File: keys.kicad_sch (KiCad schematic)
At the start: 168 parts, among them SW1 RotaryEncoder_Switch, U11 SLSS49E-3, U12 SLSS49E-3, U13 SLSS49E-3, U14 SLSS49E-3, U15 SLSS49E-3, U16 SLSS49E-3, U17 SLSS49E-3, U18 SLSS49E-3, U19 SLSS49E-3, U2 SLSS49E-3, U20 SLSS49E-3, U21 SLSS49E-3, U22 SLSS49E-3, U23 SLSS49E-3, U24 SLSS49E-3, U25 SLSS49E-3, U26 SLSS49E-3, U27 SLSS49E-3, U28 SLSS49E-3, U29 SLSS49E-3, U30 SLSS49E-3, U31 SLSS49E-3, U32 SLSS49E-3, U33 SLSS49E-3, U34 SLSS49E-3, U35 SLSS49E-3, U36 SLSS49E-3, U37 SLSS49E-3, U38 SLSS49E-3, U39 SLSS49E-3, U4 SLSS49E-3, U40 SLSS49E-3, U41 SLSS49E-3, U42 SLSS49E-3, U43 SLSS49E-3, U44 SLSS49E-3, U45 SLSS49E-3, U46 SLSS49E-3, U47 SLSS49E-3, U48 SLSS49E-3, U49 SLSS49E-3, U50 SLSS49E-3, U51 SLSS49E-3, U52 SLSS49E-3, U53 SLSS49E-3, U54 SLSS49E-3, U55 SLSS49E-3, U56 SLSS49E-3, U57 SLSS49E-3, U58 SLSS49E-3, U59 SLSS49E-3, U60 SLSS49E-3, U61 SLSS49E-3, U62 SLSS49E-3, U63 SLSS49E-3, U64 SLSS49E-3, U65 SLSS49E-3, U66 SLSS49E-3, U67 SLSS49E-3, U68 SLSS49E-3, U69 SLSS49E-3, U70 SLSS49E-3, U71 SLSS49E-3, U72 SLSS49E-3, U73 SLSS49E-3, U74 SLSS49E-3, U75 SLSS49E-3, U76 SLSS49E-3, U77 SLSS49E-3, U78 SLSS49E-3, U79 SLSS49E-3, U80 SLSS49E-3, U81 SLSS49E-3, U82 SLSS49E-3, U83 SLSS49E-3, U84 SLSS49E-3, U85 SLSS49E-3, U86 SLSS49E-3, U87 SLSS49E-3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

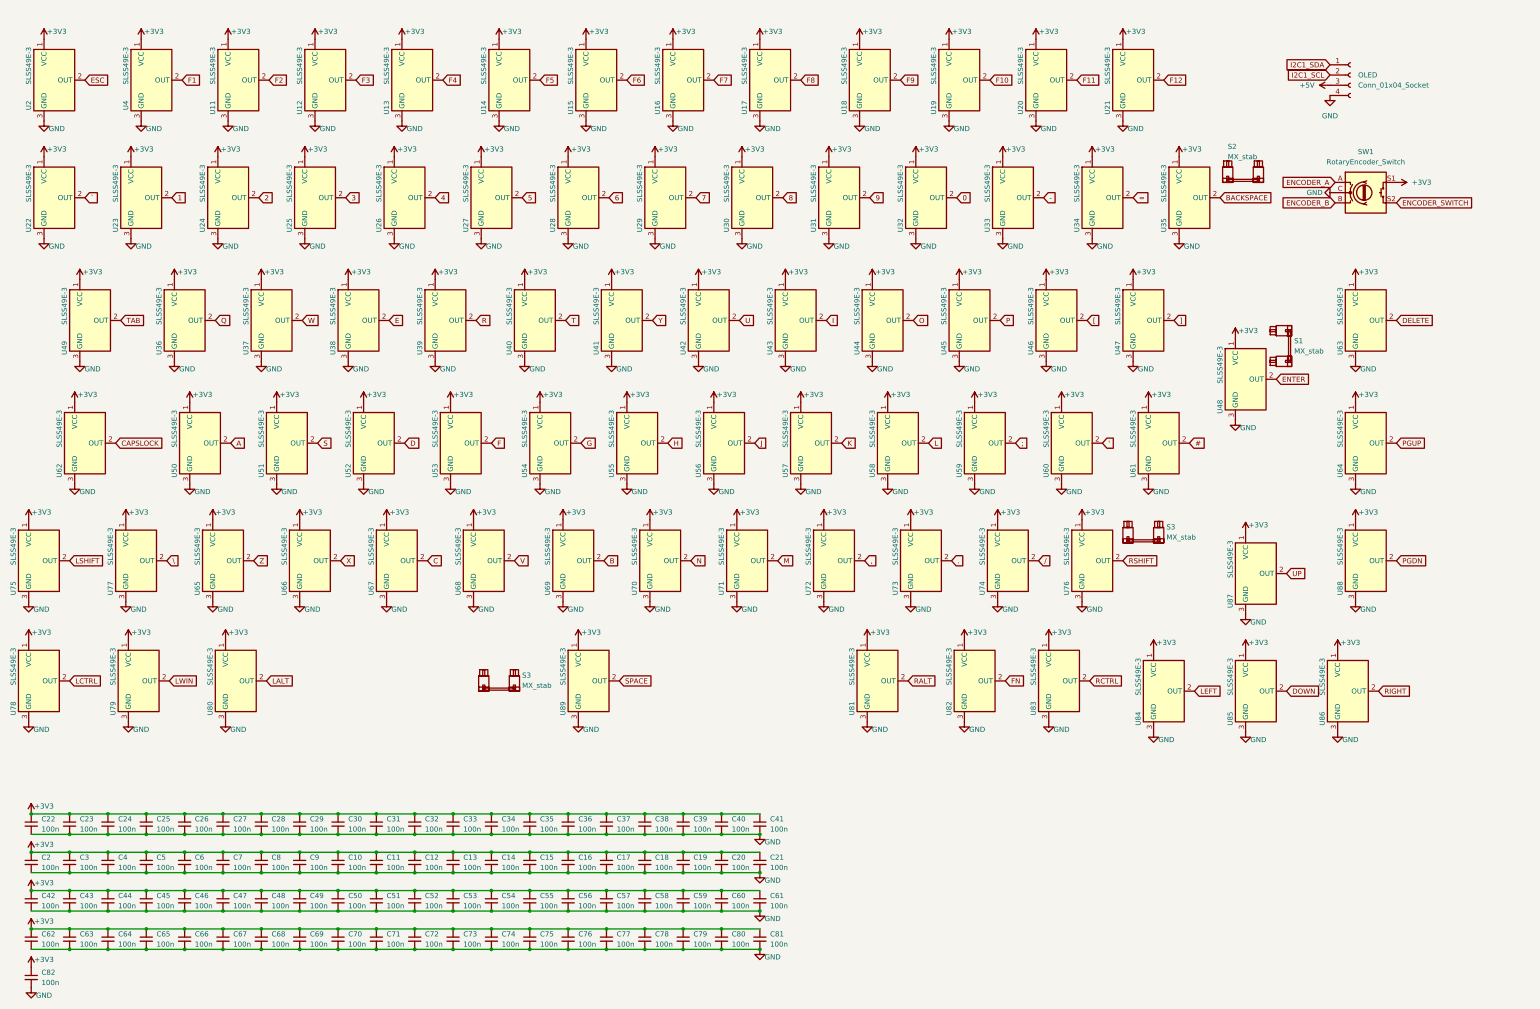
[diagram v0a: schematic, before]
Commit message: bus
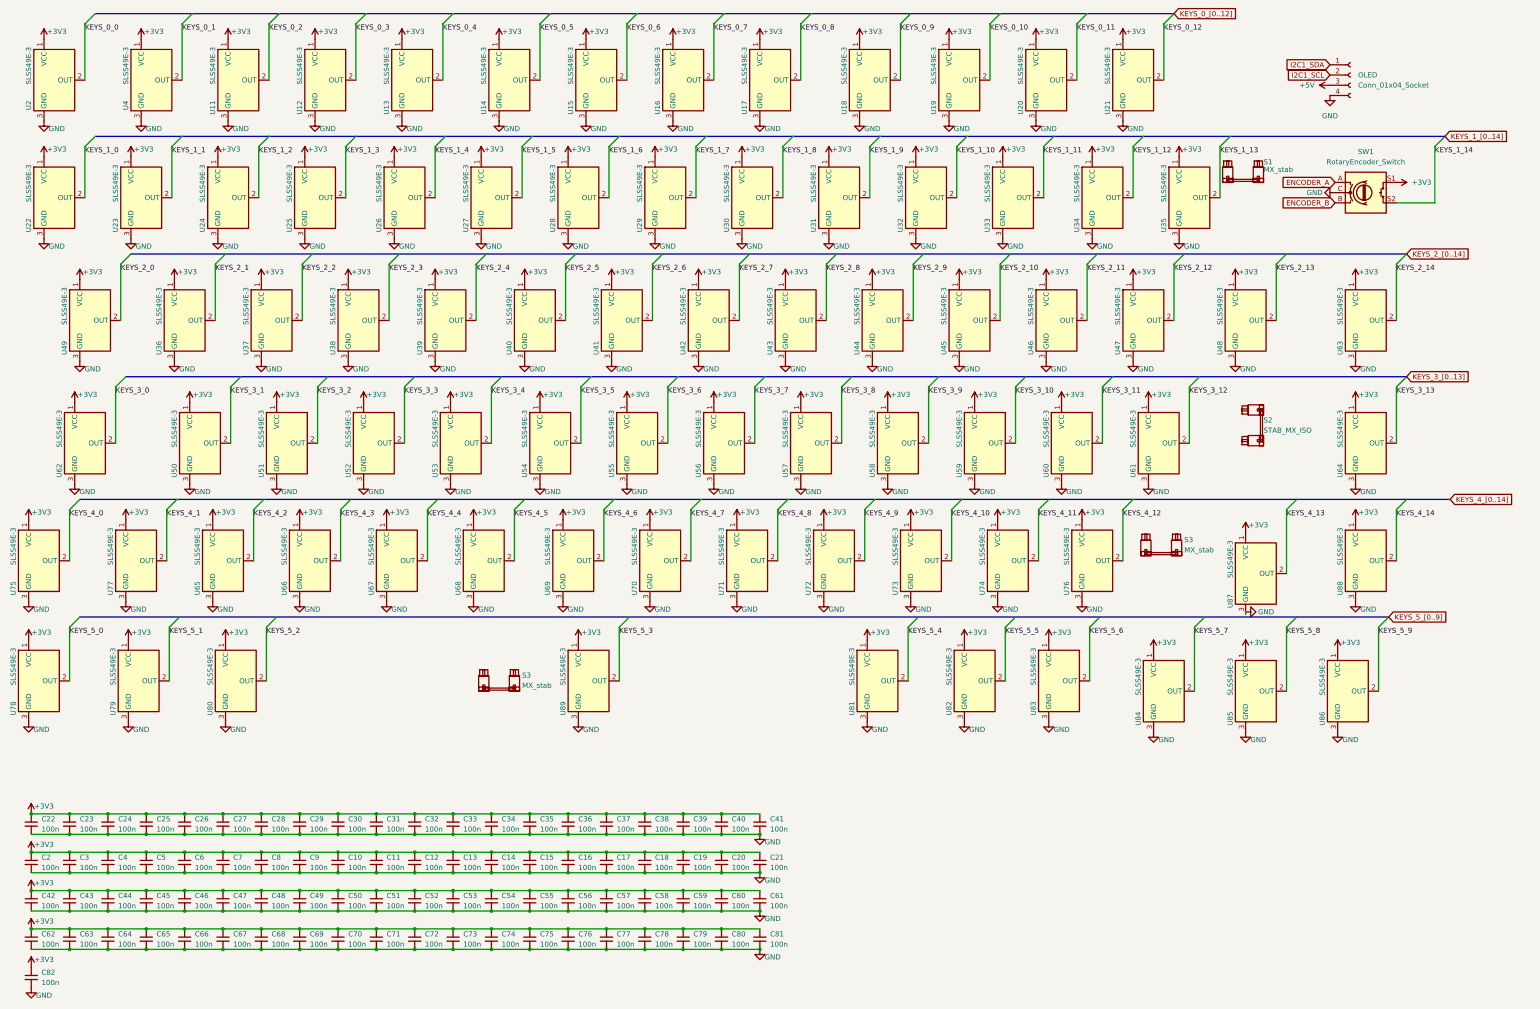
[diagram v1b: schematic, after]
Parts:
- S2: renamed from S1; value MX_stab -> STAB_MX_ISO
- renumbered S2 to S1
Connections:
- net # renamed KEYS_3_12
- net ' renamed KEYS_3_11
- net , renamed KEYS_4_9
- net - renamed KEYS_1_11
- net . renamed KEYS_4_10
- net 0 renamed KEYS_1_10
- net 1 renamed KEYS_1_1
- net 2 renamed KEYS_1_2
- net 3 renamed KEYS_1_3
- net 4 renamed KEYS_1_4
- net 5 renamed KEYS_1_5
- net 6 renamed KEYS_1_6
- net 7 renamed KEYS_1_7
- net 8 renamed KEYS_1_8
- net 9 renamed KEYS_1_9
- net ; renamed KEYS_3_10
- net = renamed KEYS_1_12
- net A renamed KEYS_3_1
- net B renamed KEYS_4_6
- net BACKSPACE renamed KEYS_1_13
- net C renamed KEYS_4_4
- net CAPSLOCK renamed KEYS_3_0
- net D renamed KEYS_3_3
- net DELETE renamed KEYS_2_14
- net DOWN renamed KEYS_5_8
- net E renamed KEYS_2_3
- net ENCODER_SWITCH renamed KEYS_1_14
- net ENTER renamed KEYS_2_13
- net ESC renamed KEYS_0_0
- net F renamed KEYS_3_4
- net F1 renamed KEYS_0_1
- net F10 renamed KEYS_0_10
- net F11 renamed KEYS_0_11
- net F12 renamed KEYS_0_12
- net F2 renamed KEYS_0_2
- net F3 renamed KEYS_0_3
- net F4 renamed KEYS_0_4
- net F5 renamed KEYS_0_5
- net F6 renamed KEYS_0_6
- net F7 renamed KEYS_0_7
- net F8 renamed KEYS_0_8
- net F9 renamed KEYS_0_9
- net FN renamed KEYS_5_5
- net G renamed KEYS_3_5
- net H renamed KEYS_3_6
- net I renamed KEYS_2_8
- net J renamed KEYS_3_7
- net K renamed KEYS_3_8
- net L renamed KEYS_3_9
- net LALT renamed KEYS_5_2
- net LCTRL renamed KEYS_5_0
- net LEFT renamed KEYS_5_7
- net LSHIFT renamed KEYS_4_0
- net LWIN renamed KEYS_5_1
- net M renamed KEYS_4_8
- net N renamed KEYS_4_7
- net O renamed KEYS_2_9
- net P renamed KEYS_2_10
- net PGDN renamed KEYS_4_14
- net PGUP renamed KEYS_3_13
- net Q renamed KEYS_2_1
- net R renamed KEYS_2_4
- net RALT renamed KEYS_5_4
- net RCTRL renamed KEYS_5_6
- net RIGHT renamed KEYS_5_9
- net RSHIFT renamed KEYS_4_12
- net S renamed KEYS_3_2
- net SPACE renamed KEYS_5_3
- net T renamed KEYS_2_5
- net TAB renamed KEYS_2_0
- net U renamed KEYS_2_7
- net UP renamed KEYS_4_13
- net V renamed KEYS_4_5
- net W renamed KEYS_2_2
- net X renamed KEYS_4_3
- net Y renamed KEYS_2_6
- net Z renamed KEYS_4_2
- net [ renamed KEYS_2_11
- net \ renamed KEYS_4_1
- net ] renamed KEYS_2_12
- net ` renamed KEYS_1_0
- net / renamed KEYS_4_11
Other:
- moved on the sheet: S2, S3, U48

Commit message: assign footprints
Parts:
- C10, C11, C12, C13, C14, C15, C16, C17, C18, C19, C2, C20, C21, C22, C23, C24, C25, C26, C27, C28, C29, C3, C30, C31, C32, C33, C34, C35, C36, C37, C38, C39, C4, C40, C41, C42, C43, C44, C45, C46, C47, C48, C49, C5, C50, C51, C52, C53, C54, C55, C56, C57, C58, C59, C6, C60, C61, C62, C63, C64, C65, C66, C67, C68, C69, C7, C70, C71, C72, C73, C74, C75, C76, C77, C78, C79, C8, C80, C81, C82, C9: footprint (none) -> Capacitor_SMD:C_0402_1005Metric
- SW1: footprint (none) -> Rotary_Encoder:RotaryEncoder_Alps_EC11E-Switch_Vertical_H20mm
- U11, U12, U13, U14, U15, U16, U17, U18, U19, U2, U20, U21, U22, U23, U24, U25, U26, U27, U28, U29, U30, U31, U32, U33, U34, U35, U36, U37, U38, U39, U4, U40, U41, U42, U43, U44, U45, U46, U47, U48, U49, U50, U51, U52, U53, U54, U55, U56, U57, U58, U59, U60, U61, U62, U63, U64, U65, U66, U67, U68, U69, U70, U71, U72, U73, U74, U75, U76, U77, U78, U79, U80, U81, U82, U83, U84, U85, U86, U87, U88, U89: footprint Package_TO_SOT_SMD:SOT-23 -> MoonBoard:SLSS49E-3 with MX holes
